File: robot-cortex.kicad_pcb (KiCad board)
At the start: 4 copper layers, 27.5 x 35.8 mm, 91 parts, among them IC1 THVD2410VDRCR, IC2 THVD2410VDRCR, IC3 THVD2410VDRCR, J1 USB4110GFA, M1 THRU_HOLE_PAD, M2 THRU_HOLE_PAD, Q1 SSM3K15F,LF, Q2 SS8050-G, U1 C2901617, U10 TPS63070, U11 TPS63070, U12 DF52-4S-0.8H(21), U13 DF52-4S-0.8H(21), U14 DF52-4S-0.8H(21), U2 STM32G431CBT6, U3 TLE9250XSJXUMA1, U4 DF52-5S-0.8H(21), U5 DF52-4S-0.8H(21), U6 SPX3819M5-L-5-0, U7 DF52-8S-0.8H(21), U8 ESP32-WROOM-32E-H4, U9 CP2102N-A02-GQFN24R

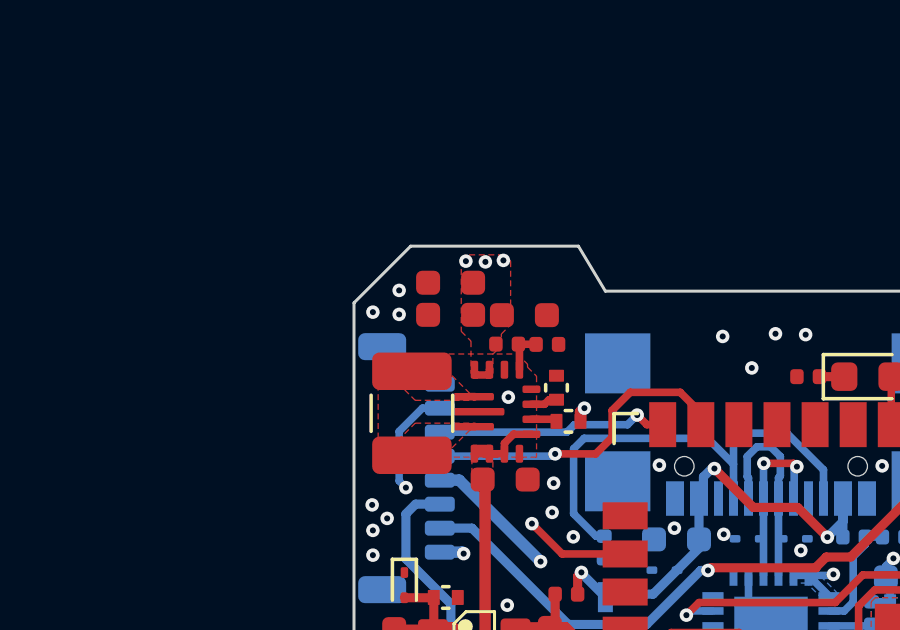
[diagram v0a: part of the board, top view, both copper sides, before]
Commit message: bom updates
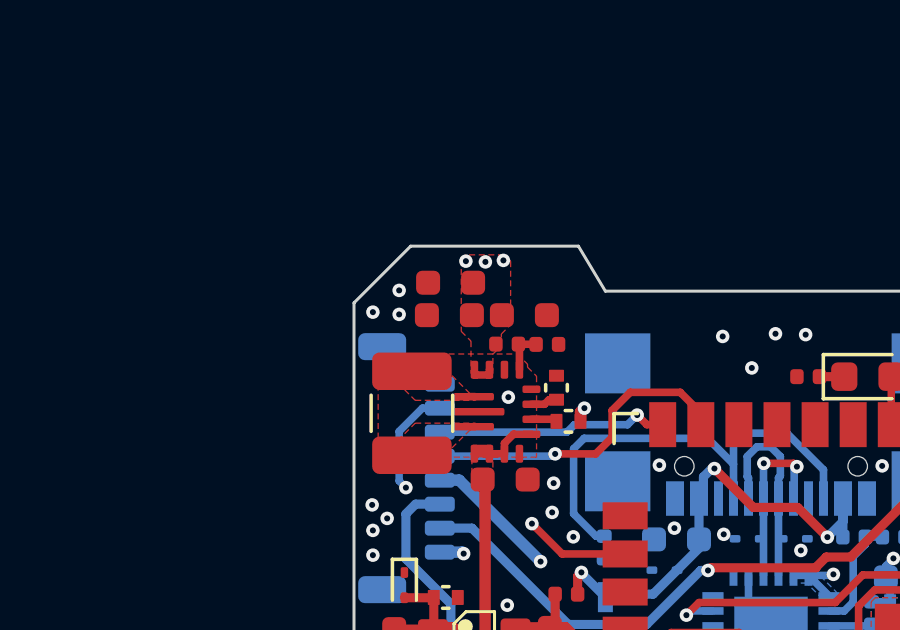
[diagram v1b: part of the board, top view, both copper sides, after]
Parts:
- C22, C25: value C386081 -> 10uF
- C24, C27, C29, C30, C32, C33: value C2998534 -> 10uF
- U4: value DF52-5S-0.8H(21) -> DF52-3S-0.8H(21)
